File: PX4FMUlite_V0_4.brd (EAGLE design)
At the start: 48.6 x 34.9 mm, 126 parts, among them J2 DF13-4P-1.25V, J201 DF13C-6P-1.25V, J202 DF13C-6P-1.25V, J203 DF13C-6P-1.25V, J3 DF13C-4P-1.25V, J302 DF13C-4P-1.25V, J401 DF13C-4P-1.25V, J403 DF13C-7P-1.25V, J405 DF13C-4P-1.25V, J802 DF13C-3P-1.25V, M3_MOUNT1101 MOUNT-HOLE3.1MM, M3_MOUNT1102 MOUNT-HOLE3.1MM, M3_MOUNT1103 MOUNT-HOLE3.1MM, M3_MOUNT1104 MOUNT-HOLE3.1MM, U101 STM32F4X7VX, U2 MAX3051, U401 MAX3051, X101 3.2x2.5 mm / 24 MHz / 15 ppm

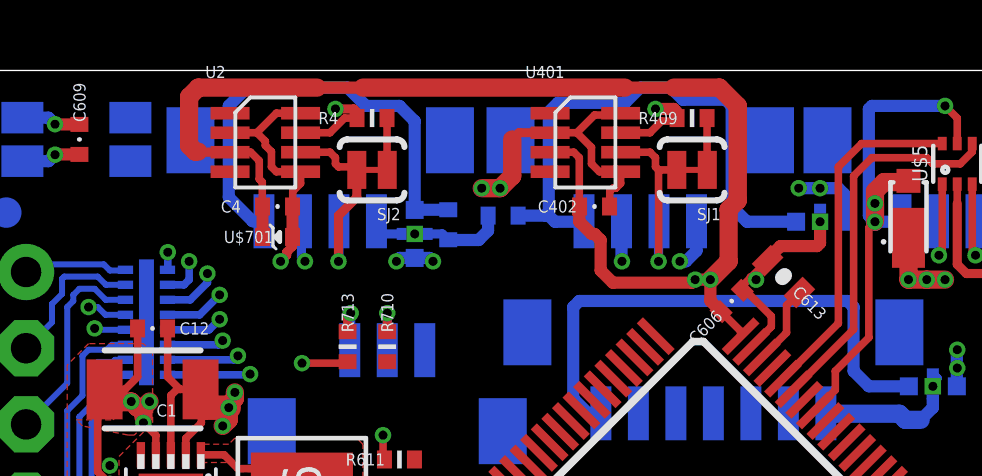
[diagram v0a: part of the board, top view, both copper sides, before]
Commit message: Tweaks tweaks
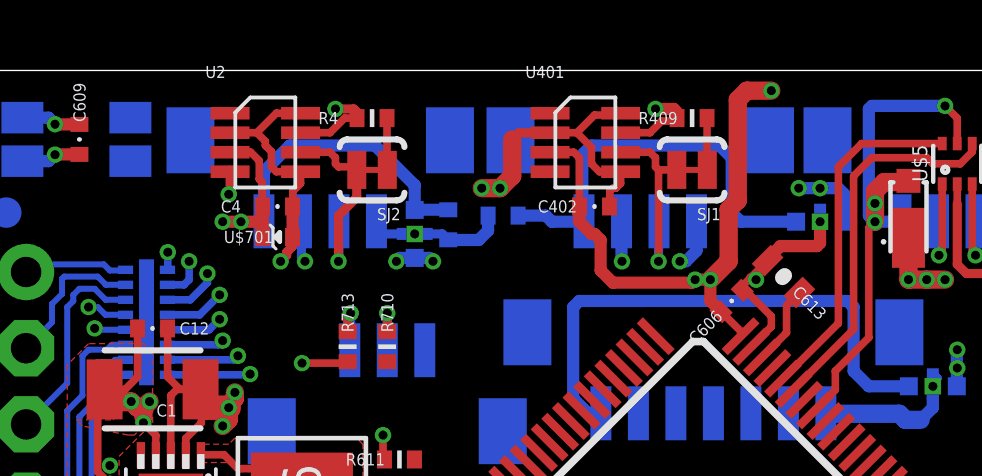
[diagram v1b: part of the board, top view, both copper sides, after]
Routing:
- net N$28: track 15.5 -> 9.54 mm
- net N$48: track 18.2 -> 13.9 mm
- net FMU-VDD_3V3: track 84.6 -> 85.8 mm, vias 11 -> 14
- net CAN2_RX: track 0.00 -> 0.81 mm, vias 0 -> 1
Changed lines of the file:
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@@
 <layer number="17" name="Pads" color="2" fill="1" visible="yes" active="yes"/>
 <layer number="18" name="Vias" color="2" fill="1" visible="yes" active="yes"/>
-<layer number="19" name="Unrouted" color="14" fill="1" visible="yes" active="yes"/>
+<layer number="19" name="Unrouted" color="14" fill="1" visible="no" active="yes"/>
 <layer number="20" name="Dimension" color="15" fill="1" visible="yes" active="yes"/>
 <layer number="21" name="tPlace" color="7" fill="1" visible="yes" active="yes"/>
@@
 <wire x1="39.4208" y1="31.2928" x2="39.4208" y2="33.02" width="0.6096" layer="1"/>
 <wire x1="39.4208" y1="33.02" x2="39.7256" y2="33.3248" width="0.6096" layer="1"/>
-<wire x1="39.7256" y1="33.3248" x2="39.7256" y2="36.4744" width="0.6096" layer="1"/>
-<wire x1="39.7256" y1="36.4744" x2="39.116" y2="37.084" width="0.6096" layer="1"/>
-<wire x1="39.116" y1="37.084" x2="37.592" y2="37.084" width="0.6096" layer="1"/>
-<wire x1="37.592" y1="37.084" x2="35.9664" y2="37.084" width="0.4064" layer="1"/>
-<wire x1="35.9664" y1="37.084" x2="27.2288" y2="37.084" width="0.6096" layer="1"/>
-<wire x1="27.2288" y1="37.084" x2="25.7048" y2="37.084" width="0.4064" layer="1"/>
-<wire x1="25.7048" y1="37.084" x2="21.7424" y2="37.084" width="0.6096" layer="1"/>
-<wire x1="21.7424" y1="37.084" x2="21.4376" y2="36.7792" width="0.6096" layer="1"/>
-<wire x1="21.4376" y1="36.7792" x2="21.4376" y2="35.1536" width="0.6096" layer="1"/>
-<wire x1="21.4376" y1="35.1536" x2="21.6408" y2="34.9504" width="0.6096" layer="1"/>
-<wire x1="21.6408" y1="34.9504" x2="21.7424" y2="34.9504" width="0.6096" layer="1"/>
-<wire x1="21.7424" y1="34.9504" x2="21.7626" y2="34.9302" width="0.3048" layer="1"/>
-<wire x1="21.7626" y1="34.9302" x2="22.8026" y2="34.9302" width="0.3048" layer="1"/>
+<wire x1="39.7256" y1="33.3248" x2="39.7256" y2="36.6776" width="0.6096" layer="1"/>
 <via x="38.8112" y="30.6832" extent="1-16" drill="0.3"/>
 <via x="38.3032" y="30.6832" extent="1-16" drill="0.3"/>
@@
 <wire x1="39.360128125" y1="10.8712" x2="40.52611875" y2="9.705209375" width="0.254" layer="1"/>
 <wire x1="37.2872" y1="11.3792" x2="37.592" y2="11.684" width="0.254" layer="1"/>
-<wire x1="23.884" y1="32.1056" x2="23.884" y2="33.1216" width="0.4064" layer="1"/>
+<wire x1="23.884" y1="32.1056" x2="23.884" y2="32.6136" width="0.4064" layer="1"/>
+<wire x1="23.884" y1="32.6136" x2="23.884" y2="33.1216" width="0.4064" layer="1"/>
 <wire x1="34.4424" y1="33.1216" x2="34.4424" y2="32.6136" width="0.4064" layer="1"/>
 <wire x1="34.4424" y1="32.6136" x2="34.8488" y2="32.2072" width="0.4064" layer="1"/>
@@
 <wire x1="27.2288" y1="19.1944" x2="27.948" y2="19.1944" width="0.254" layer="16"/>
 <wire x1="27.948" y1="19.1944" x2="28.0416" y2="19.1008" width="0.254" layer="16"/>
+<wire x1="39.7256" y1="36.6776" x2="40.0304" y2="36.9824" width="0.6096" layer="1"/>
+<wire x1="40.0304" y1="36.9824" x2="40.8432" y2="36.9824" width="0.6096" layer="1"/>
+<via x="40.8432" y="36.9824" extent="1-16" drill="0.3"/>
+<wire x1="40.8432" y1="36.9824" x2="37.8968" y2="36.9824" width="0.6096" layer="15"/>
+<wire x1="37.8968" y1="36.9824" x2="37.7952" y2="37.084" width="0.4064" layer="15"/>
+<wire x1="37.7952" y1="37.084" x2="36.4744" y2="37.084" width="0.4064" layer="15"/>
+<wire x1="36.4744" y1="37.084" x2="36.3728" y2="36.9824" width="0.4064" layer="15"/>
+<wire x1="36.3728" y1="36.9824" x2="28.2528" y2="36.9824" width="0.6096" layer="15"/>
+<wire x1="28.2528" y1="36.9824" x2="23.884" y2="32.6136" width="0.6096" layer="15"/>
+<wire x1="23.884" y1="32.6136" x2="23.1648" y2="32.6136" width="0.6096" layer="15"/>
+<via x="22.5552" y="32.6136" extent="1-16" drill="0.3"/>
+<wire x1="23.1648" y1="32.6136" x2="22.5552" y2="32.6136" width="0.6096" layer="15"/>
+<wire x1="22.5552" y1="32.6136" x2="23.1648" y2="32.6136" width="0.4064" layer="1"/>
+<wire x1="23.1648" y1="32.6136" x2="23.884" y2="32.6136" width="0.4064" layer="1"/>
 <wire x1="48.6664" y1="18.6944" x2="50.792" y2="21.2344" width="0" layer="19" extent="1-15"/>
 <wire x1="29.2916" y1="28.332" x2="27.948" y2="22.9616" width="0" layer="19" extent="1-16"/>
 <wire x1="40.3352" y1="21.844" x2="39.8190125" y2="28.79709375" width="0" layer="19" extent="1-16"/>
+<via x="23.1648" y="32.6136" extent="1-16" drill="0.3"/>
 </signal>
 <signal name="OTG_FS_DP">
@@
 <contactref element="U101" pad="51"/>
 <contactref element="U2" pad="4"/>
-<wire x1="22.8026" y1="34.2802" x2="48.30429375" y2="20.3118125" width="0" layer="19" extent="1-1"/>
+<wire x1="22.8026" y1="34.2802" x2="22.7584" y2="34.2802" width="0.4064" layer="1"/>
+<via x="22.7584" y="33.528" extent="1-16" drill="0.3"/>
+<wire x1="22.7584" y1="33.528" x2="22.8026" y2="33.5722" width="0.3048" layer="1"/>
+<wire x1="22.8026" y1="33.5722" x2="22.8026" y2="34.2802" width="0.3048" layer="1"/>
+<wire x1="22.8026" y1="33.5722" x2="48.30429375" y2="20.3118125" width="0" layer="19" extent="1-1"/>
 </signal>
 <signal name="CAN2_TX">
@@
 <contactref element="R408" pad="P$1"/>
 <wire x1="37.092" y1="5.588" x2="36.3728" y2="5.588" width="0.4064" layer="1"/>
-<wire x1="36.3728" y1="5.588" x2="34.5157125" y2="11.472978125" width="0" layer="19" extent="1-16"/>
 <via x="36.3728" y="5.588" extent="1-16" drill="0.3"/>
+<wire x1="36.3728" y1="5.588" x2="34.5157125" y2="11.472978125" width="0" layer="19" extent="1-1"/>
 </signal>
 <signal name="FMU_AUX_ADC2">
@@
 <contactref element="R407" pad="P$1"/>
 <wire x1="41.648" y1="5.588" x2="42.164" y2="5.588" width="0.4064" layer="1"/>
-<wire x1="42.164" y1="5.588" x2="42.293884375" y2="11.472978125" width="0" layer="19" extent="1-16"/>
 <via x="42.164" y="5.588" extent="1-16" drill="0.3"/>
+<wire x1="42.164" y1="5.588" x2="42.293884375" y2="11.472978125" width="0" layer="19" extent="1-1"/>
 </signal>
 <signal name="N$68">
@@
 <contactref element="L403" pad="P$2"/>
 <contactref element="U$404" pad="C"/>
-<wire x1="39.3192" y1="36.6776" x2="37.8968" y2="36.6776" width="0.4064" layer="16"/>
-<wire x1="37.8968" y1="36.6776" x2="37.4904" y2="37.084" width="0.4064" layer="16"/>
-<wire x1="37.4904" y1="37.084" x2="36.4744" y2="37.084" width="0.4064" layer="16"/>
-<wire x1="36.4744" y1="37.084" x2="35.9664" y2="36.576" width="0.4064" layer="16"/>
-<wire x1="35.9664" y1="36.576" x2="33.7312" y2="36.576" width="0.4064" layer="16"/>
-<wire x1="33.7312" y1="36.576" x2="33.4264" y2="36.2712" width="0.4064" layer="16"/>
-<wire x1="33.4264" y1="36.2712" x2="33.4264" y2="32.9184" width="0.4064" layer="16"/>
-<wire x1="33.4264" y1="32.9184" x2="33.4264" y2="32.8168" width="0.4064" layer="16"/>
-<wire x1="33.4264" y1="32.8168" x2="33.6296" y2="32.6136" width="0.4064" layer="16"/>
-<wire x1="33.6296" y1="32.6136" x2="34.585" y2="32.6136" width="0.4064" layer="16"/>
+<wire x1="41.6688" y1="32.6136" x2="39.8272" y2="32.6136" width="0.4064" layer="16"/>
+<wire x1="39.8272" y1="32.6136" x2="39.5224" y2="32.9184" width="0.4064" layer="16"/>
+<wire x1="39.5224" y1="32.9184" x2="39.5224" y2="34.7472" width="0.4064" layer="16"/>
+<wire x1="39.5224" y1="34.7472" x2="39.116" y2="35.1536" width="0.4064" layer="16"/>
+<wire x1="39.116" y1="35.1536" x2="34.8488" y2="35.1536" width="0.4064" layer="16"/>
+<wire x1="34.8488" y1="35.1536" x2="34.544" y2="34.8488" width="0.4064" layer="16"/>
+<wire x1="34.544" y1="34.8488" x2="34.544" y2="32.6834" width="0.4064" layer="16"/>
+<wire x1="34.544" y1="32.6834" x2="34.5994" y2="32.628" width="0.4064" layer="16"/>
+<wire x1="32.4024" y1="32.8168" x2="33.3248" y2="32.8168" width="0.4064" layer="16"/>
+<wire x1="33.3248" y1="32.8168" x2="33.528" y2="32.6136" width="0.4064" layer="16"/>
+<wire x1="33.528" y1="32.6136" x2="34.585" y2="32.6136" width="0.4064" layer="16"/>
 <wire x1="34.585" y1="32.6136" x2="34.5994" y2="32.628" width="0.4064" layer="16"/>
-<wire x1="32.4024" y1="32.8168" x2="33.3248" y2="32.8168" width="0.4064" layer="16"/>
-<wire x1="33.3248" y1="32.8168" x2="33.4264" y2="32.9184" width="0.4064" layer="16"/>
-<wire x1="39.3192" y1="36.6776" x2="39.5352" y2="36.4616" width="0.4064" layer="16"/>
-<wire x1="39.5352" y1="36.4616" x2="39.5224" y2="36.4616" width="0.4064" layer="16"/>
-<wire x1="39.5224" y1="36.4616" x2="39.5224" y2="33.1216" width="0.4064" layer="16"/>
-<wire x1="39.5224" y1="33.1216" x2="40.0304" y2="32.6136" width="0.4064" layer="16"/>
-<wire x1="40.0304" y1="32.6136" x2="41.6688" y2="32.6136" width="0.4064" layer="16"/>
 </signal>
 <signal name="5V_S3_FILTERED" class="1">
@@
 <contactref element="L7" pad="P$2"/>
 <contactref element="U$7" pad="C"/>
-<wire x1="28.956" y1="33.0072" x2="28.956" y2="35.9664" width="0.4064" layer="16"/>
-<wire x1="28.956" y1="35.9664" x2="28.448" y2="36.4744" width="0.4064" layer="16"/>
-<wire x1="28.448" y1="36.4744" x2="27.3304" y2="36.4744" width="0.4064" layer="16"/>
-<wire x1="27.3304" y1="36.4744" x2="26.7208" y2="37.084" width="0.4064" layer="16"/>
-<wire x1="26.7208" y1="37.084" x2="23.368" y2="37.084" width="0.4064" layer="16"/>
-<wire x1="23.368" y1="37.084" x2="22.7584" y2="36.4744" width="0.4064" layer="16"/>
-<wire x1="22.7584" y1="36.4744" x2="22.7584" y2="33.4264" width="0.4064" layer="16"/>
-<wire x1="22.7584" y1="33.4264" x2="23.5568" y2="32.628" width="0.4064" layer="16"/>
-<wire x1="23.5568" y1="32.628" x2="23.9314" y2="32.628" width="0.4064" layer="16"/>
 <wire x1="30.0736" y1="33.012" x2="28.9608" y2="33.012" width="0.4064" layer="16"/>
 <wire x1="28.9608" y1="33.012" x2="28.956" y2="33.0072" width="0.4064" layer="16"/>
+<wire x1="28.956" y1="33.0072" x2="28.956" y2="33.8328" width="0.4064" layer="16"/>
+<wire x1="28.956" y1="33.8328" x2="27.6352" y2="35.1536" width="0.4064" layer="16"/>
+<wire x1="27.6352" y1="35.1536" x2="24.7904" y2="35.1536" width="0.4064" layer="16"/>
+<wire x1="24.7904" y1="35.1536" x2="23.9314" y2="34.2946" width="0.4064" layer="16"/>
+<wire x1="23.9314" y1="34.2946" x2="23.9314" y2="32.628" width="0.4064" layer="16"/>
 </signal>
 <signal name="N$29">
